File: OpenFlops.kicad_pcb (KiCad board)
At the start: 2 copper layers, 111.6 x 59.4 mm, 87 parts, among them J99 OSHW_LOGO, P1 FLOPPY_CONN, P2 POWER_INPUT, P3 USB_A_FEMALE, P4 PROG_PORT, P5 JUMPER_JC, P6 ENCODER_PORT, P7 DISPLAY_PORT, P8 USB_HEADER, P9 EXTERNAL_SPEAKER, Q1 BSS138, Q2 BSS138, Q3 BSS138, Q4 BSS138, Q5 BSS138, Q6 BSS138, Q7 MMBT3904, U1 74HCT04, U3 STM32F105RBT6, U4 LM1117-3.3, Y1 8 MHz

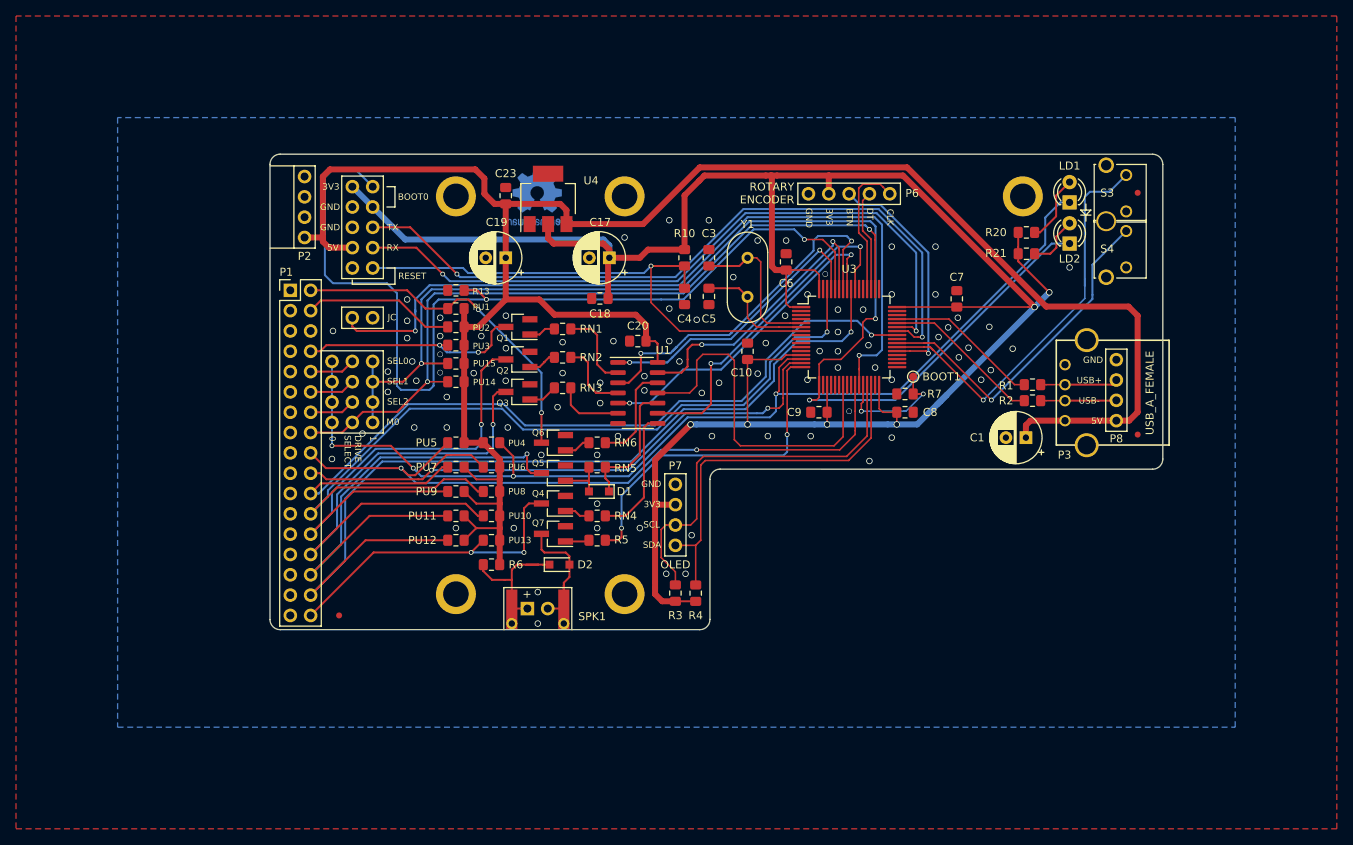
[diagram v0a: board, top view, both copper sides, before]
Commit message: Restructure for v1.0 or the Ferguson version
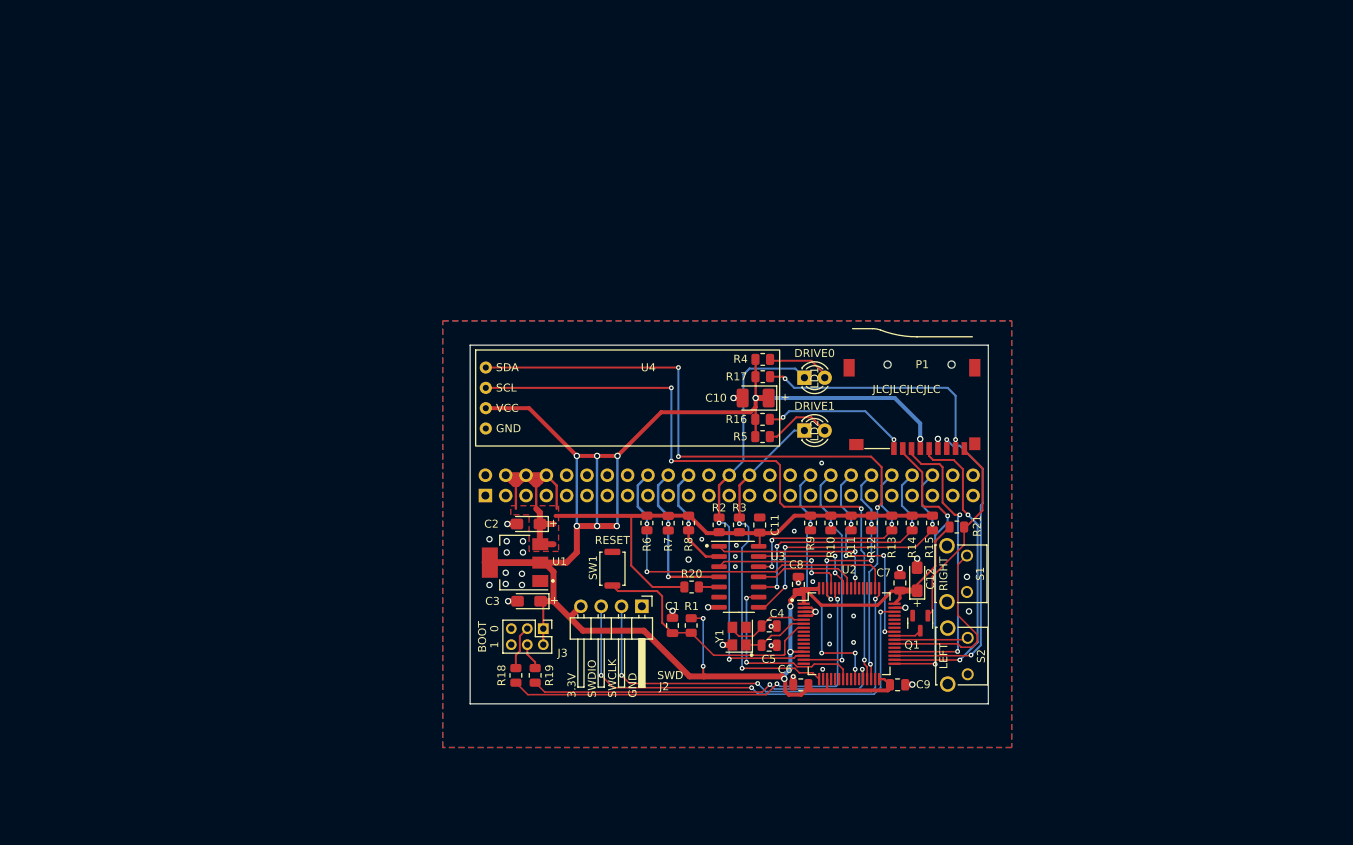
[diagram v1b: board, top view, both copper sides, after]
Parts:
- removed C17, C19: 10u, Capacitor_THT:CP_Radial_D6.3mm_P2.50mm
- removed C18, C20, C23: 100n, Capacitor_SMD:C_0805_2012Metric_Pad1.15x1.40mm_HandSolder
- removed D1, D2: 1N4148, Diode_SMD:D_SOD-323_HandSoldering
- removed FID1, FID2, FID3: Fiducial, Fiducial:Fiducial_0.75mm_Mask1.5mm
- removed H1, H2, H3, H4, H5: MountingHole_Pad, OpenFlops:MountingHole_M3_Pad
- removed J99: OSHW_LOGO, Symbol:OSHW-Logo2_9.8x8mm_Copper
- removed P2: POWER_INPUT, OpenFlops:PinHeader_1x04_P2.54mm_Vertical
- removed P3: USB_A_FEMALE, OpenFlops:USB_A_FEMALE
- removed P4: PROG_PORT, OpenFlops:PinHeader_2x05_P2.54mm_Vertical
- removed P5: JUMPER_JC, OpenFlops:PinHeader_1x02_P2.54mm_Vertical
- removed P6: ENCODER_PORT, OpenFlops:PinHeader_1x05_P2.54mm_Vertical
- removed P7: DISPLAY_PORT, OpenFlops:PinHeader_1x04_P2.54mm_Vertical
- removed P8: USB_HEADER, OpenFlops:PinHeader_1x04_P2.54mm_Vertical
- removed P9: EXTERNAL_SPEAKER, OpenFlops:PinHeader_1x02_P2.54mm_Mute
- removed PA5, PB5, PC5, PD5: Conn_01x03, OpenFlops:PinHeader_1x03_P2.54mm_Mute
- removed PU1, PU10, PU11, PU12, PU13, PU14, PU15, PU2, PU3, PU4, PU5, PU6, PU7, PU8, PU9: 1k, Resistor_SMD:R_0805_2012Metric_Pad1.15x1.40mm_HandSolder
- removed Q2, Q3, Q4, Q5, Q6: BSS138, Package_TO_SOT_SMD:SOT-23_Handsoldering
- removed Q7: MMBT3904, Package_TO_SOT_SMD:SOT-23_Handsoldering
- removed RN1, RN2, RN3, RN4, RN5, RN6: 1K, Resistor_SMD:R_0805_2012Metric_Pad1.15x1.40mm_HandSolder
- removed S3: BT_RIGHT, OpenFlops:PUSH_BUTTON_RIGHT_ANGLE
- removed S4: BT_LEFT, OpenFlops:PUSH_BUTTON_RIGHT_ANGLE
- removed SPK1: Speaker, OpenFlops:Buzzer
- removed TP1: BOOT1, TestPoint:TestPoint_Pad_D1.0mm
- added C11: 100n, Capacitor_SMD:C_0805_2012Metric, F.Cu at (156.5, 101.7)
- added C12: 22uf, Capacitor_Tantalum_SMD:CP_EIA-3216-12_Kemet-S_Pad1.58x1.35mm_HandSolder, F.Cu at (176.1, 108.5)
- added C2: 22uf, Capacitor_Tantalum_SMD:CP_EIA-3216-12_Kemet-S_Pad1.58x1.35mm_HandSolder, F.Cu at (127.5, 101.6)
- added J1: Conn_02x25_Odd_Even, Connector_PinSocket_2.54mm:PinSocket_2x25_P2.54mm_Vertical, B.Cu at (122.2, 98.0)
- added J2: SWD, Connector_PinHeader_2.54mm:PinHeader_1x04_P2.54mm_Horizontal, F.Cu at (141.7, 111.9)
- added J3: BOOT 1/0, Connector_PinHeader_2.00mm:PinHeader_2x03_P2.00mm_Vertical, F.Cu at (129.4, 114.7)
- added R11: 1K, Resistor_SMD:R_0805_2012Metric, F.Cu at (167.9, 101.5)
- added R12: 1K, Resistor_SMD:R_0805_2012Metric, F.Cu at (170.4, 101.5)
- added R14: 1K, Resistor_SMD:R_0805_2012Metric, F.Cu at (175.5, 101.5)
- added R15: 1K, Resistor_SMD:R_0805_2012Metric, F.Cu at (178.1, 101.5)
- added R16: 10K, Resistor_SMD:R_0805_2012Metric, F.Cu at (156.8, 88.5)
- added R17: 10K, Resistor_SMD:R_0805_2012Metric, F.Cu at (156.8, 83.2)
- added R18: 10K, Resistor_SMD:R_0805_2012Metric, F.Cu at (126.0, 120.5)
- added R19: 10K, Resistor_SMD:R_0805_2012Metric, F.Cu at (128.4, 120.5)
- added R8: 1K, Resistor_SMD:R_0805_2012Metric, F.Cu at (147.6, 101.5)
- added R9: 1K, Resistor_SMD:R_0805_2012Metric, F.Cu at (162.8, 101.5)
- added S1: RIGHT, OpenFlops:PUSH_BUTTON_RIGHT_ANGLE, F.Cu at (182.4, 107.8)
- added S2: LEFT, OpenFlops:PUSH_BUTTON_RIGHT_ANGLE, F.Cu at (182.5, 118.1)
- added SW1: RESET, Button_Switch_SMD:SW_Push_SPST_NO_Alps_SKRK, F.Cu at (138.0, 107.2)
- added U2: AT32F435RGT7, Package_QFP:LQFP-64_10x10mm_P0.5mm, F.Cu at (167.6, 115.3)
- C1: value 100u -> 100n; footprint Capacitor_THT:CP_Radial_D6.3mm_P2.50mm -> Capacitor_SMD:C_0805_2012Metric
- C10: value 100n -> 47uf; footprint Capacitor_SMD:C_0805_2012Metric_Pad1.15x1.40mm_HandSolder -> Capacitor_Tantalum_SMD:CP_EIA-3528-12_Kemet-T_Pad1.50x2.35mm_HandSolder
- C3: value 22p -> 22uf; footprint Capacitor_SMD:C_0805_2012Metric_Pad1.15x1.40mm_HandSolder -> Capacitor_Tantalum_SMD:CP_EIA-3216-12_Kemet-S_Pad1.58x1.35mm_HandSolder
- C4: value 100n -> 22p; footprint Capacitor_SMD:C_0805_2012Metric_Pad1.15x1.40mm_HandSolder -> Capacitor_SMD:C_0805_2012Metric
- C5, C6, C7, C8, C9: footprint Capacitor_SMD:C_0805_2012Metric_Pad1.15x1.40mm_HandSolder -> Capacitor_SMD:C_0805_2012Metric
- LD1: value LED_GREEN -> DRIVE0
- LD2: value LED_RED -> DRIVE1
- P1: value FLOPPY_CONN -> ST-TF-003A; footprint Connector_PinHeader_2.54mm:PinHeader_2x17_P2.54mm_Vertical -> ST-TF-003A:SUNTECH_ST-TF-003A
- Q1: footprint Package_TO_SOT_SMD:SOT-23_Handsoldering -> Package_TO_SOT_SMD:SOT-23
- R1: value 22 -> 4k7; footprint Resistor_SMD:R_0805_2012Metric_Pad1.15x1.40mm_HandSolder -> Resistor_SMD:R_0805_2012Metric
- R10, R13, R7: value 4k7 -> 1K; footprint Resistor_SMD:R_0805_2012Metric_Pad1.15x1.40mm_HandSolder -> Resistor_SMD:R_0805_2012Metric
- R2: value 22 -> 1k; footprint Resistor_SMD:R_0805_2012Metric_Pad1.15x1.40mm_HandSolder -> Resistor_SMD:R_0805_2012Metric
- R20, R21: value 1k -> 10K; footprint Resistor_SMD:R_0805_2012Metric_Pad1.15x1.40mm_HandSolder -> Resistor_SMD:R_0805_2012Metric
- R3, R4: value 3.3K -> 1k; footprint Resistor_SMD:R_0805_2012Metric_Pad1.15x1.40mm_HandSolder -> Resistor_SMD:R_0805_2012Metric
- R5: value 1K -> 1k; footprint Resistor_SMD:R_0805_2012Metric_Pad1.15x1.40mm_HandSolder -> Resistor_SMD:R_0805_2012Metric
- R6: value 22 -> 1K; footprint Resistor_SMD:R_0805_2012Metric_Pad1.15x1.40mm_HandSolder -> Resistor_SMD:R_0805_2012Metric
- U1: value 74HCT04 -> LM1117-3.3; footprint Package_SO:SOIC-14_3.9x8.7mm_P1.27mm -> Package_TO_SOT_SMD:SOT-223-3_TabPin2
- U3: value STM32F105RBT6 -> 74LS07; footprint OpenFlops:LQFP-64_Handsoldering -> Package_SO:SOIC-14_3.9x8.7mm_P1.27mm
- U4: value LM1117-3.3 -> OLED-0.91-128x32; footprint Package_TO_SOT_SMD:SOT-223-3_TabPin2 -> Tersteeg:OLED-0.91-128x32
- Y1: value 8 MHz -> 8MHz; footprint Crystal:Crystal_HC49-U_Vertical -> Crystal:Crystal_SMD_Abracon_ABM8G-4Pin_3.2x2.5mm
- moved P1 80.3 mm to (176.8, 86.8), turned to 180 degrees
- moved Q1 62.5 mm to (176.5, 114.0), turned to -90 degrees
- moved R13 61.8 mm to (173.0, 101.5), turned to -90 degrees
- moved R20 61.0 mm to (148.0, 109.5), turned to 0 degrees
- moved C6 52.9 mm to (161.6, 121.7), turned to 180 degrees
- moved R1 52.2 mm to (147.9, 114.3), turned to -90 degrees
- moved C1 50.0 mm to (145.6, 114.3), turned to 90 degrees
- moved C3 48.5 mm to (127.6, 111.3), turned to 180 degrees
- moved Y1 47.3 mm to (153.9, 115.6), turned to 90 degrees
- moved C5 44.3 mm to (157.7, 116.8), turned to 0 degrees
- moved C4 42.5 mm to (157.7, 114.3), turned to 0 degrees
- moved R2 42.1 mm to (151.4, 101.7), turned to -90 degrees
- moved LD2 40.6 mm to (162.0, 89.9), turned to 0 degrees
- moved LD1 39.7 mm to (162.1, 83.3), turned to 0 degrees
- moved R10 37.9 mm to (165.4, 101.5)
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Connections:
- C1 pad 1: +5V -> /nrst
- C3 pad 1: Net-(C3-Pad1) -> +3V3
- C4 pad 1: /nrst -> Net-(U2-PD0)
- C5 pad 1: Net-(C5-Pad1) -> Net-(U2-PD1)
- LD1 pad 1: /~selx -> /~{sel0}
- LD1 pad 2: Net-(LD1-Pad2) -> Net-(LD1-A)
- LD2 pad 1: /~sely -> /~{sel1}
- LD2 pad 2: Net-(LD2-Pad2) -> Net-(LD2-A)
- P1 pad 1: GND -> Net-(P1-DAT2)
- P1 pad 2: /~dskchg -> /spi_cs
- P1 pad 3: GND -> /spi_di
- P1 pad 4: /~inuse -> +3V3
- P1 pad 5: GND -> /spi_clk
- P1 pad 6: (no net) -> GND
- P1 pad 7: GND -> /spi_do
- P1 pad 8: /~index -> Net-(P1-DAT1)
- P1 pad 9: GND -> /cd_socket
- Q1 pad 1: Net-(Q1-Pad1) -> /cd_socket
- Q1 pad 3: /~index -> /cd
- R1 pad 1: /usb+r -> +3V3
- R1 pad 2: /usb+ -> /nrst
- R10 pad 1: +3V3 -> +5V
- R10 pad 2: /nrst -> /~{step}
- R13 pad 1: /boot0 -> +5V
- R13 pad 2: GND -> /~{trk0}
- R2 pad 1: /usb-r -> /~{sel0}
- R2 pad 2: /usb- -> +5V
- R20 pad 1: Net-(LD1-Pad2) -> +5V
- R20 pad 2: +3V3 -> Net-(R20-Pad2)
- R21 pad 1: Net-(LD2-Pad2) -> +3V3
- R21 pad 2: +3V3 -> /cd_socket
- R3 pad 1: +3V3 -> /~{sel1}
- R3 pad 2: /disp_clk -> +5V
- R4 pad 1: +3V3 -> Net-(LD1-A)
- R4 pad 2: /disp_dio -> +3V3
- R5 pad 1: Net-(Q7-Pad1) -> Net-(LD2-A)
- R5 pad 2: /jb -> +3V3
- R6 pad 1: /spk+ -> +5V
- R6 pad 2: +5V -> /~{mtron}
- R7 pad 1: GND -> +5V
- R7 pad 2: /boot1 -> /~{index}
- U1 pad 1: /~index_3v3 -> GND
- U1 pad 2: Net-(RN1-Pad2) -> +3V3
- U1 pad 3: /~trk0_3v3 -> +5V
- U3 pad 1: +3V3 -> /~{rdy_3v3}
- U3 pad 10: (no net) -> /~{wprot}
- U3 pad 11: (no net) -> /~{wprot_3v3}
- U3 pad 12: GND -> /~{trk0}
- U3 pad 13: +3V3 -> /~{trk0_3v3}
- U3 pad 14: /~selx -> +5V
- U3 pad 2: GND -> /~{rdy}
- U3 pad 3: GND -> /~{index_3v3}
- U3 pad 4: GND -> /~{index}
- U3 pad 5: Net-(C3-Pad1) -> Net-(R20-Pad2)
- U3 pad 6: Net-(C5-Pad1) -> unconnected-(U3-Pad6)
- U3 pad 7: /nrst -> GND
- U3 pad 8: (no net) -> /~{rdata}
- U3 pad 9: (no net) -> /~{rdata_3v3}
- U4 pad 3: +5V -> /disp_clk
- Y1 pad 1: Net-(C3-Pad1) -> Net-(U2-PD1)
- Y1 pad 2: Net-(C5-Pad1) -> GND
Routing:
- net /~sely: track 154.9 -> 0.00 mm, vias 3 -> 0
- net +5V: track 256.2 -> 103.0 mm
- net /~selx: track 133.6 -> 0.00 mm, vias 4 -> 0
- net /~side: track 111.9 -> 0.00 mm, vias 1 -> 0
- net /~wgate: track 106.8 -> 0.00 mm, vias 1 -> 0
- net /~wdata: track 104.9 -> 0.00 mm, vias 1 -> 0
- net /jc: track 99.9 -> 0.00 mm, vias 2 -> 0
- net /~mtron: track 97.4 -> 0.00 mm, vias 2 -> 0
- net /tx: track 91.1 -> 0.00 mm, vias 2 -> 0
- net /rx: track 87.9 -> 0.00 mm, vias 2 -> 0
- net /~step: track 78.5 -> 0.00 mm, vias 2 -> 0
- net /boot0: track 119.5 -> 53.9 mm
- net /~wprot: track 64.0 -> 0.00 mm, vias 1 -> 0
- net /~rdata: track 60.9 -> 0.00 mm, vias 1 -> 0
- net /~trk0: track 59.3 -> 0.00 mm, vias 1 -> 0
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- added copper zone on F.Cu, net +5V
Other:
- board size 111.6 x 59.4 mm -> 64.8 x 44.8 mm
- net class Default removed
- net class Power removed
- net class uC removed
- board text added: "3.3V"
- board text added: "BOOT"
- board text added: "FlashFloppy for Ferguson v1.0 PCB by Chris Tersteeg github.com/djtersteegc/OpenFlops-Ferguson"
- board text added: "JLCJLCJLCJLC"
- board text added: "SWCLK"
- board text added: "SWDIO"
- board text removed: "3V3"
- board text removed: "5V"
- board text removed: "BOOT0"
- board text removed: "BOOT1"
- board text removed: "BTN"
- board text removed: "CLK"
- board text removed: "DRIVE SELECT"
- board text removed: "DT"
- board text removed: "JC"
- board text removed: "Licensed under CERN OHL v.1.2"
- board text removed: "M0"
- board text removed: "OLED"
- board text removed: "RESET"
- board text removed: "ROTARY ENCODER"
- board text removed: "RX"
- board text removed: "SCL"
- board text removed: "SDA"
- board text removed: "SEL0"
- board text removed: "SEL1"
- board text removed: "SEL2"
- board text removed: "TX"
- board text removed: "USB+"
- board text removed: "USB-"
- board text removed: "V1"
- board text removed: "github.com/SukkoPera/OpenFlops"
